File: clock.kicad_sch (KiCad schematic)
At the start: 47 parts, among them J1 Conn_01x03_Pin, J11 HLT, SW1 Step, SW2 Clk Source, SW2 Run / Step, SW4 RESET, U1 LM555, U2 LM555, U3 LM555, U4 74LS04, U5 74LS08, U6 74LS32, U7 LM555, X1 ACO-xxxMHz

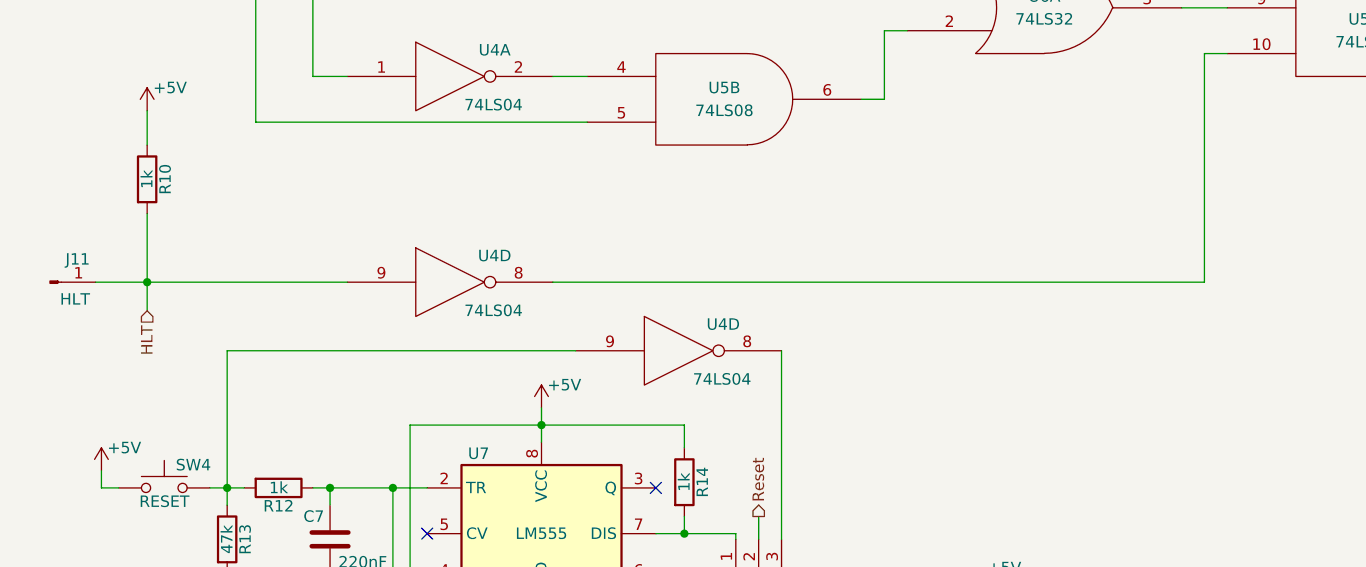
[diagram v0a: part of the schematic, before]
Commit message: Fix Oops...
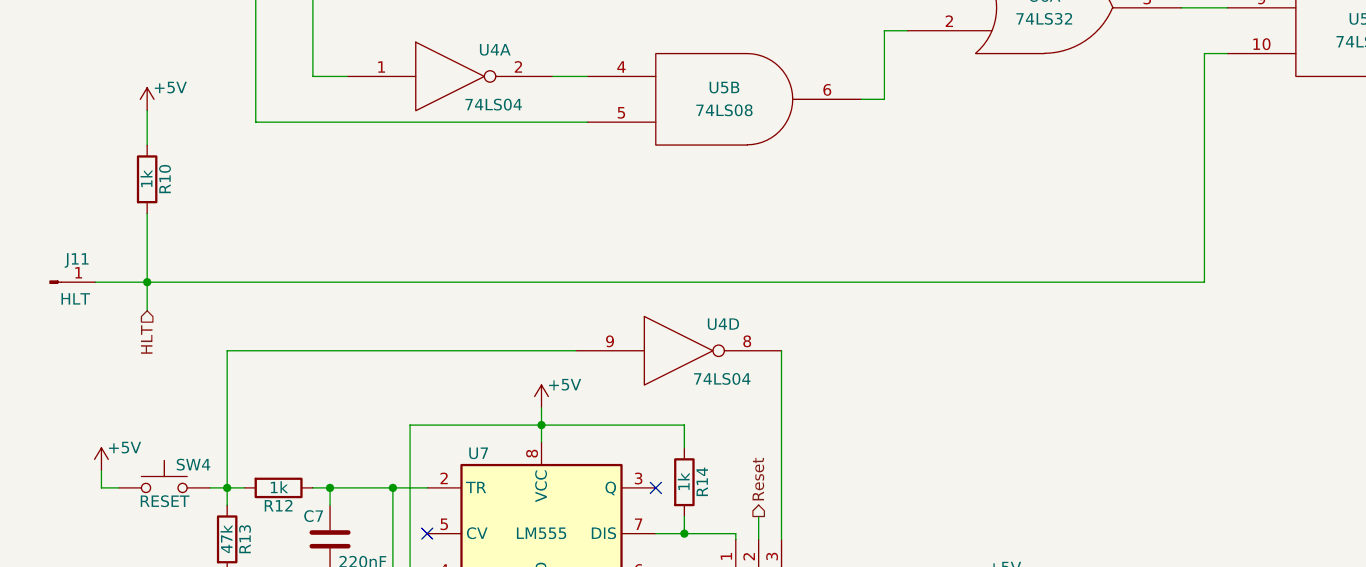
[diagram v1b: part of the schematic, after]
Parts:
- removed U4: 74LS04, Package_DIP:DIP-14_W7.62mm, symbol 8bit-computer-rescue:74LS04-8bit-computer-rescue
- J1: footprint Connector_PinSocket_1.27mm:PinSocket_1x03_P1.27mm_Vertical -> Connector_PinSocket_2.54mm:PinSocket_1x03_P2.54mm_Vertical
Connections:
- net HLT: now also U5.10
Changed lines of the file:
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@@
 	(wire
 		(pts
-			(xy 42.545 147.32) (xy 64.77 147.32)
+			(xy 42.545 147.32) (xy 160.02 147.32)
 		)
 		(stroke
@@
 	(wire
 		(pts
-			(xy 87.63 147.32) (xy 160.02 147.32)
-		)
-		(stroke
-			(width 0)
-			(type default)
-		)
-	)
-	(wire
-		(pts
 			(xy 39.37 77.47) (xy 50.8 77.47)
 		)
@@
 	(symbol
 		(lib_id "8bit-computer-rescue:74LS04-8bit-computer-rescue")
-		(at 76.2 147.32 0)
-		(unit 4)
-		(exclude_from_sim no)
-		(in_bom yes)
-		(on_board yes)
-		(dnp no)
-		(property "Reference" "U4"
-			(at 81.153 144.399 0)
-			(effects
-				(font
-					(size 1.27 1.27)
-				)
-			)
-		)
-		(property "Value" "74LS04"
-			(at 81.026 150.495 0)
-			(effects
-				(font
-					(size 1.27 1.27)
-				)
-			)
-		)
-		(property "Footprint" "Package_DIP:DIP-14_W7.62mm"
-			(at 76.2 147.32 0)
-			(effects
-				(font
-					(size 1.27 1.27)
-				)
-				(hide yes)
-			)
-		)
-		(property "Datasheet" ""
-			(at 76.2 147.32 0)
-			(effects
-				(font
-					(size 1.27 1.27)
-				)
-				(hide yes)
-			)
-		)
-		(property "Description" ""
-			(at 76.2 147.32 0)
-			(effects
-				(font
-					(size 1.27 1.27)
-				)
-				(hide yes)
-			)
-		)
-		(pin "14"
-		)
-		(pin "7"
-		)
-		(pin "1"
-		)
-		(pin "2"
-		)
-		(pin "3"
-		)
-		(pin "4"
-		)
-		(pin "5"
-		)
-		(pin "6"
-		)
-		(pin "8"
-		)
-		(pin "9"
-		)
-		(pin "10"
-		)
-		(pin "11"
-		)
-		(pin "12"
-		)
-		(pin "13"
-		)
-		(instances
-			(project "8bit-computer"
-				(path "/0e1a93c4-fdde-4b8f-a97d-016b71cdd04f/00000000-0000-0000-0000-00005b533ecb"
-					(reference "U4")
-					(unit 4)
-				)
-			)
-			(project "BenEater-6502"
-				(path "/64020bd5-bae0-49a1-9410-23726bcfaf48/5a49408d-bc6d-4641-a815-21b24906e7e4"
-					(reference "U4")
-					(unit 3)
-				)
-			)
-		)
-	)
-	(symbol
-		(lib_id "8bit-computer-rescue:74LS04-8bit-computer-rescue")
 		(at 223.52 107.95 0)
 		(unit 6)
@@
 			)
 		)
-		(property "Footprint" "Connector_PinSocket_1.27mm:PinSocket_1x03_P1.27mm_Vertical"
+		(property "Footprint" "Connector_PinSocket_2.54mm:PinSocket_1x03_P2.54mm_Vertical"
 			(at 110.49 180.975 0)
 			(effects
